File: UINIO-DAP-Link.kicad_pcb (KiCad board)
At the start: 2 copper layers, 100.7 x 33.3 mm, 33 parts, among them J1 扩展板串口 & 电源输出, J2 扩展板 JTAG 输出, J3 JTAG_nTRST 跳线选择, J4 3.3V 跳线选择, J5 扩展板 SWD 输入, J6 DAPLink 固件下载接口, J7 JTAG/SWD 下载接口, U1 ME6211, U2 STM32F103C8T6, Y1 Crystal_GND24

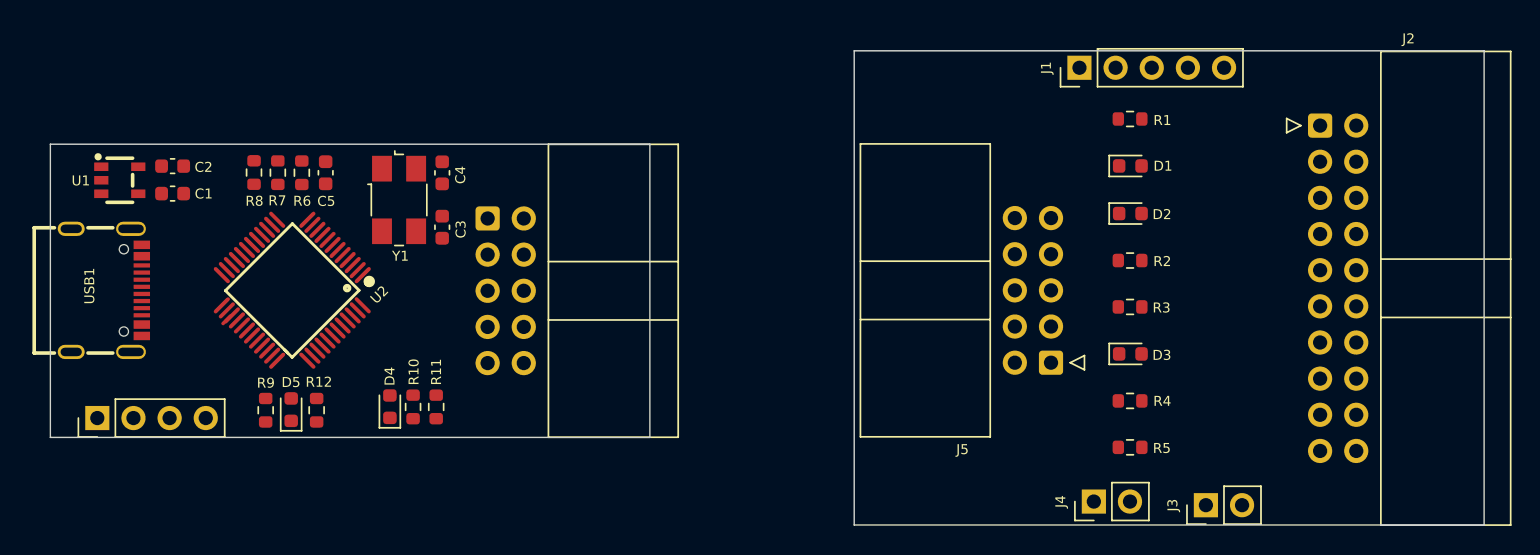
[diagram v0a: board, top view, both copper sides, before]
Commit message: Update PCB layout.
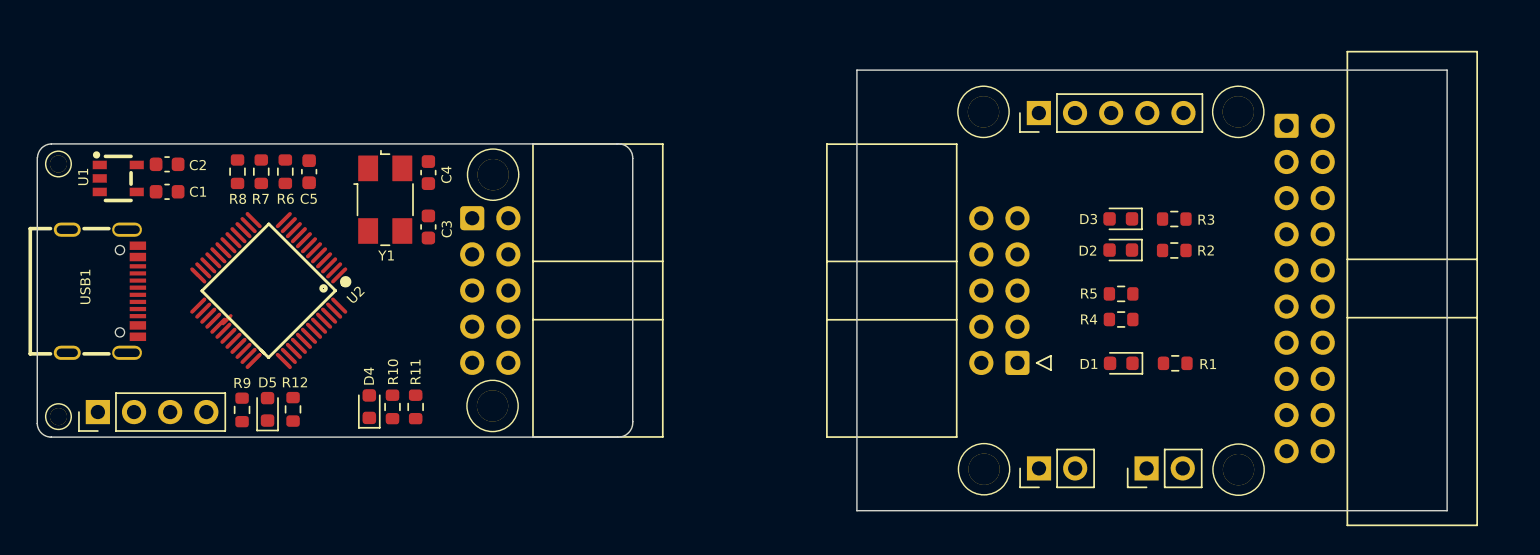
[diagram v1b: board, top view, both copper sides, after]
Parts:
- added HOLE**: Hole-1mm, Uinio:Hole-1mm, F.Cu at (33.5, 105.0)
- added HOLE**: Hole-2mm, Uinio:Hole-2mm, F.Cu at (116.4, 83.6)
- added HOLE**: Hole-2mm, Uinio:Hole-2mm, F.Cu at (116.4, 108.7)
- added HOLE**: Hole-1mm, Uinio:Hole-1mm, F.Cu at (33.5, 87.2)
- added HOLE**: Hole-2mm, Uinio:Hole-2mm, F.Cu at (98.5, 108.7)
- added HOLE**: Hole-2mm, Uinio:Hole-2mm, F.Cu at (64.0, 88.0)
- added HOLE**: Hole-2mm, Uinio:Hole-2mm, F.Cu at (98.5, 83.6)
- added HOLE**: Hole-2mm, Uinio:Hole-2mm, F.Cu at (64.0, 104.2)
- moved R1 17.5 mm to (112.0, 101.3), turned to 180 degrees
- moved D1 13.9 mm to (108.2, 101.3), turned to 180 degrees
- moved R5 10.8 mm to (108.2, 96.4), turned to 180 degrees
- moved D3 9.51 mm to (108.1, 91.1), turned to 180 degrees
- moved R3 6.92 mm to (111.9, 91.1)
- moved R4 5.75 mm to (108.2, 98.2), turned to 180 degrees
- moved J3 4.90 mm to (110.0, 108.6)
- moved J4 4.50 mm to (102.4, 108.6)
- moved J1 4.27 mm to (102.4, 83.7)
- moved R2 3.19 mm to (111.9, 93.3)
- moved D2 2.65 mm to (108.1, 93.3), turned to 180 degrees
- moved J2 2.36 mm to (119.8, 84.6)
- moved J5 2.36 mm to (100.9, 101.2)
- moved R12 1.66 mm to (50.0, 104.5)
- moved D5 1.66 mm to (48.2, 104.5)
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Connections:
- net /VTref renamed /3.3V_Output
- J5 pad 1: Net-(J5-Pad1) -> /_USART2_TX
- J5 pad 10: /_JTAG_TCK/SWCLK -> /_VDD_5V
- J5 pad 2: Net-(J5-Pad2) -> /_JTAG_TCK/SWCLK
- J5 pad 3: /_JTAG_nTRST_Output -> /_USART2_RX
- J5 pad 4: /_USART2_RX -> GND
- J5 pad 5: /_USART2_TX -> /_JTAG_nTRST_Output
- J5 pad 6: /_VDD_5V -> /_JTAG_TMS/SWDIO
- J5 pad 7: /_VDD_3.3V -> Net-(R4-Pad2)
- J5 pad 8: /_JTAG_TMS/SWDIO -> /_VDD_3.3V
- J5 pad 9: GND -> Net-(R5-Pad2)
- J7 pad 1: /USART2_TX -> /JTAG_TDI
- J7 pad 10: /VDD_5V -> /JTAG_TCK/SWCLK
- J7 pad 2: /USART2_RX -> /VDD_5V
- J7 pad 3: /JTAG_nTRST -> /JTAG_TDO
- J7 pad 4: /JTAG_TDO -> /VDD_3.3V
- J7 pad 5: /JTAG_TDI -> /JTAG_nTRST
- J7 pad 6: /JTAG_TCK/SWCLK -> /JTAG_TMS/SWDIO
- J7 pad 7: GND -> /USART2_RX
- J7 pad 8: /JTAG_TMS/SWDIO -> GND
- J7 pad 9: /VDD_3.3V -> /USART2_TX
- R4 pad 2: Net-(J5-Pad2) -> Net-(R4-Pad2)
- R5 pad 2: Net-(J5-Pad1) -> Net-(R5-Pad2)
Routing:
- net unconnected-(U2-Pad29): track 0.00 -> 0.77 mm
- net /JTAG_TMS/SWDIO: track 0.77 -> 0.00 mm
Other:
- board size 100.7 x 33.3 mm -> 99.1 x 31 mm
